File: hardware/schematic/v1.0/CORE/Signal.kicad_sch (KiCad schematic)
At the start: 13 parts, among them J2 Conn_Coaxial, J26 Conn_01x04_Socket, J3 Conn_Coaxial, J4 Conn_Coaxial, J5 Conn_Coaxial, U10 IPEX1, U11 IPEX1, U4 IPEX1, U8 IPEX1, U9 IPEX1

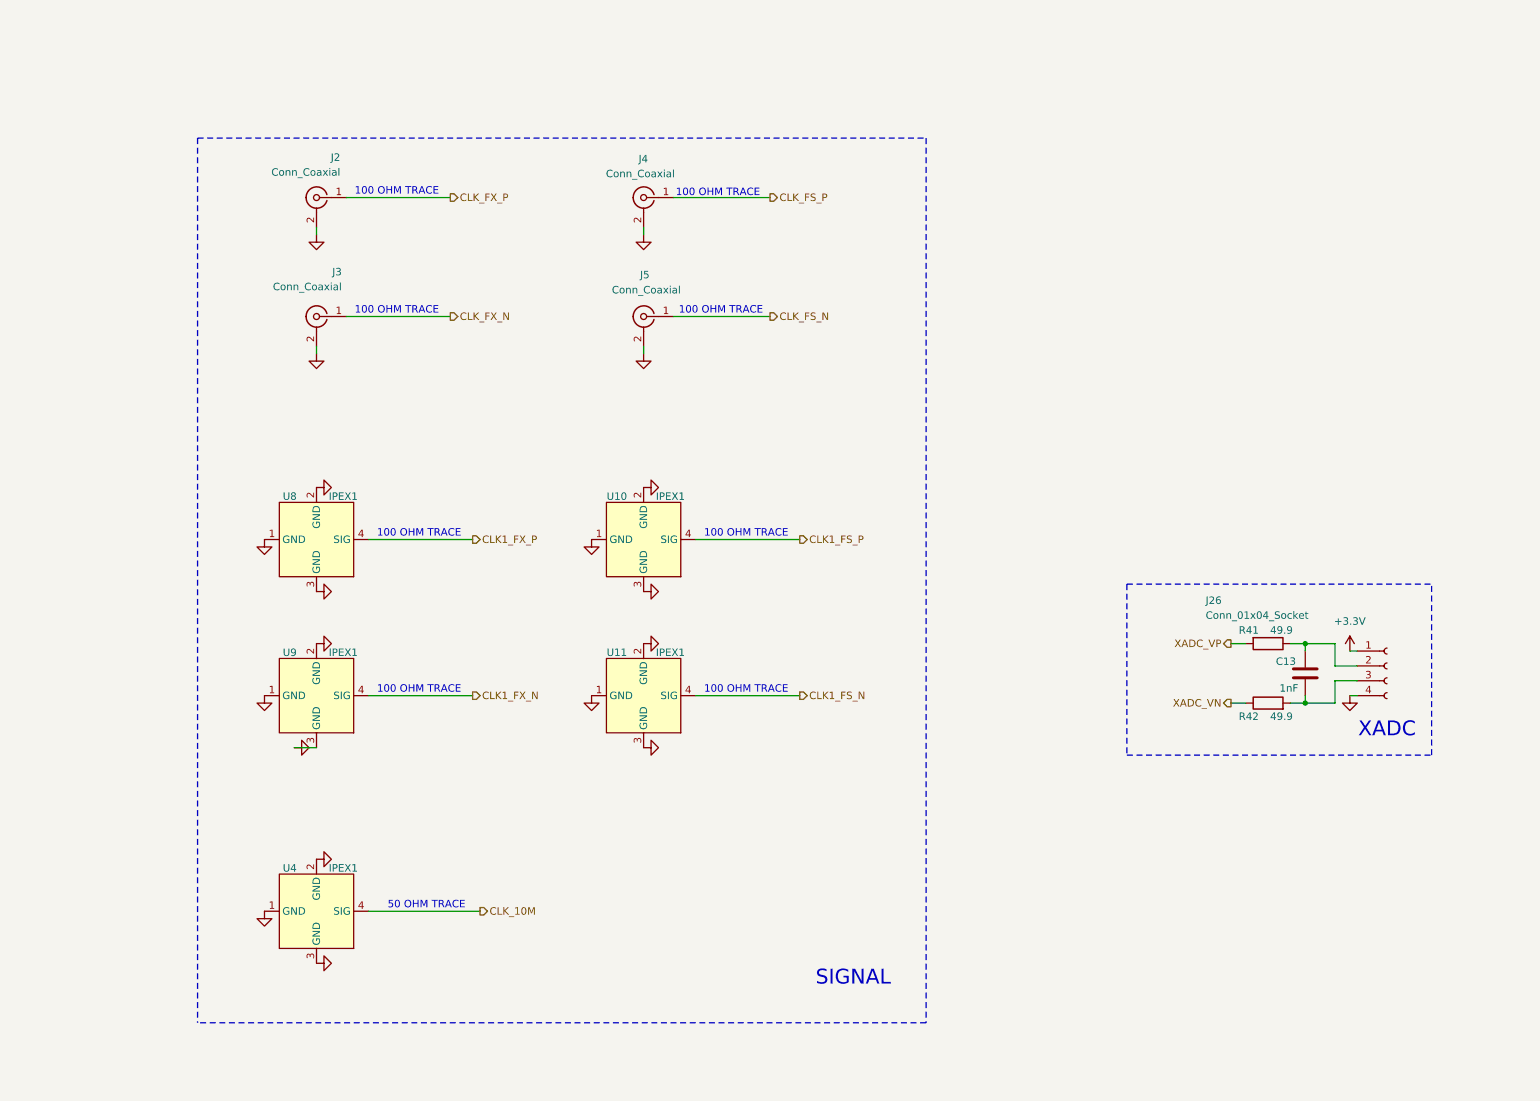
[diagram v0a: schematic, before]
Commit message: sch update
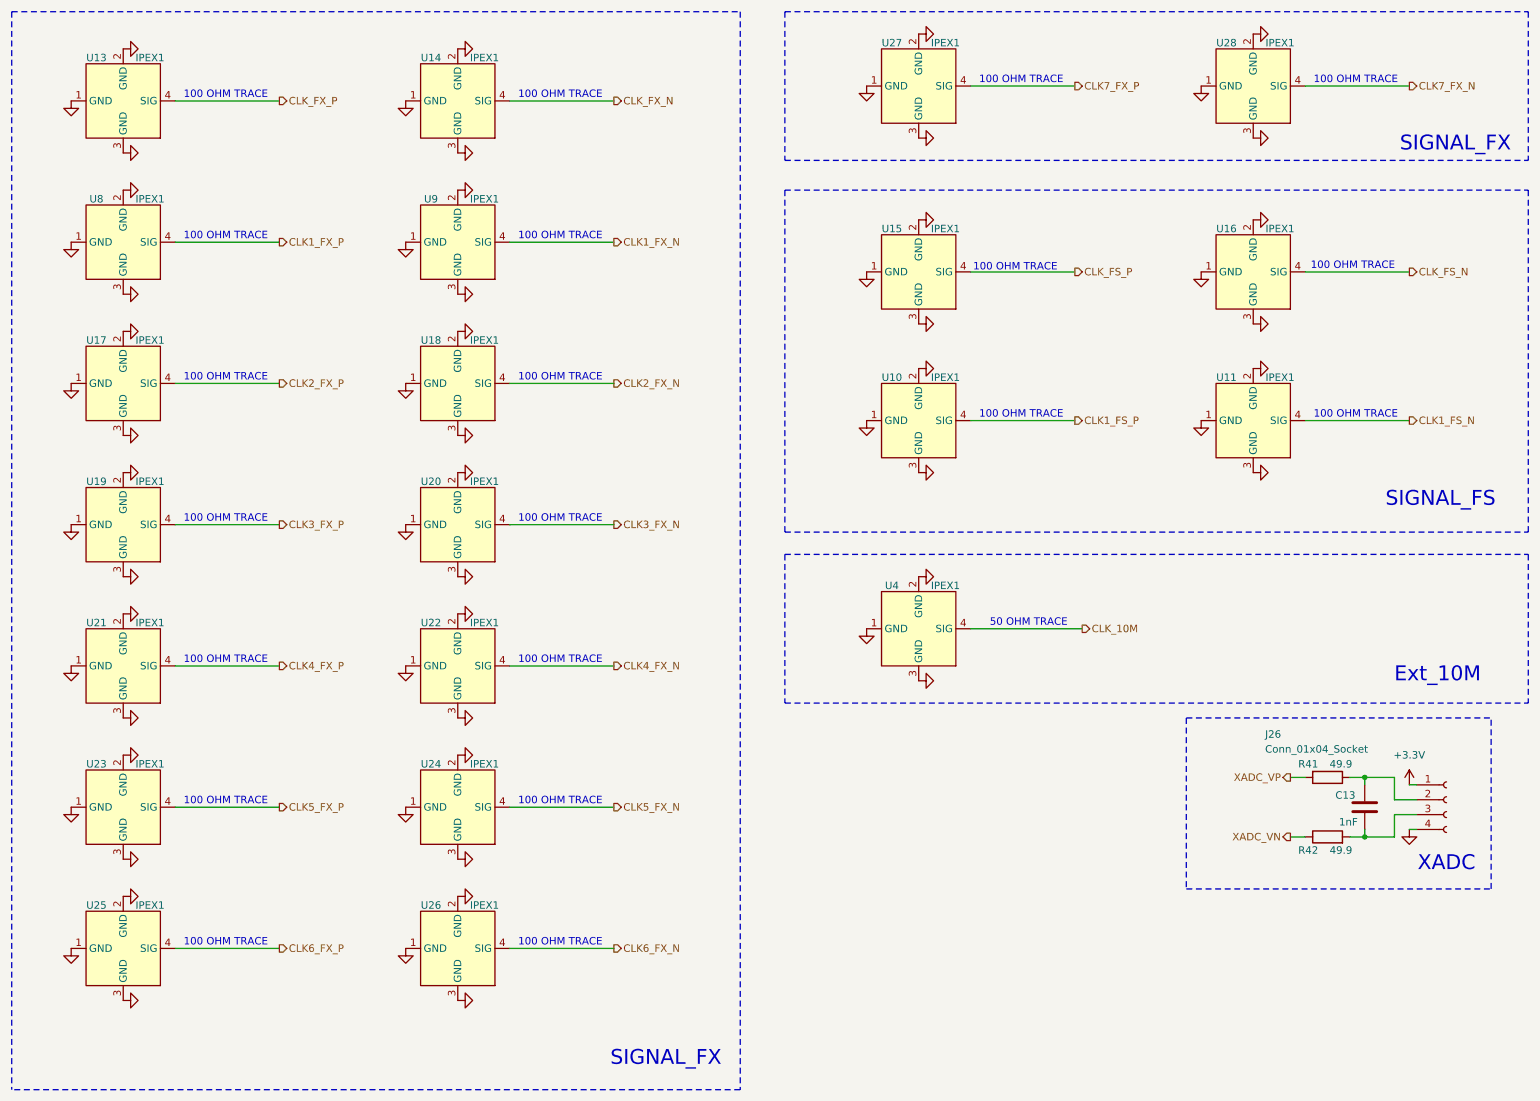
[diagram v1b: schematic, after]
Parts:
- removed J2, J3, J4, J5: Conn_Coaxial, Connector_Coaxial:SMA_Amphenol_132289_EdgeMount, symbol Connector:Conn_Coaxial
- added U13, U14, U15, U16, U17, U18, U19, U20, U21, U22, U23, U24, U25, U26, U27, U28: IPEX1, Counter:JLC_IPEX-1, symbol Counter:IPEX1
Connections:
- net CLK_FS_N: now also U16.4 (SIG)
- net CLK_FS_P: now also U15.4 (SIG)
- net CLK_FX_N: now also U14.4 (SIG)
- net CLK_FX_P: now also U13.4 (SIG)
- net GND: now also U13.1 (GND), U13.2 (GND), U13.3 (GND), U14.1 (GND), U14.2 (GND), U14.3 (GND), U15.1 (GND), U15.2 (GND), U15.3 (GND), U16.1 (GND), U16.2 (GND), U16.3 (GND), U17.1 (GND), U17.2 (GND), U17.3 (GND), U18.1 (GND), U18.2 (GND), U18.3 (GND), U19.1 (GND), U19.2 (GND), U19.3 (GND), U20.1 (GND), U20.2 (GND), U20.3 (GND), U21.1 (GND), U21.2 (GND), U21.3 (GND), U22.1 (GND), U22.2 (GND), U22.3 (GND), U23.1 (GND), U23.2 (GND), U23.3 (GND), U24.1 (GND), U24.2 (GND), U24.3 (GND), U25.1 (GND), U25.2 (GND), U25.3 (GND), U26.1 (GND), U26.2 (GND), U26.3 (GND), U27.1 (GND), U27.2 (GND), U27.3 (GND), U28.1 (GND), U28.2 (GND), U28.3 (GND)
- new net CLK2_FX_N: U18.4 (SIG)
- new net CLK2_FX_P: U17.4 (SIG)
- new net CLK3_FX_N: U20.4 (SIG)
- new net CLK3_FX_P: U19.4 (SIG)
- new net CLK4_FX_N: U22.4 (SIG)
- new net CLK4_FX_P: U21.4 (SIG)
- new net CLK5_FX_N: U24.4 (SIG)
- new net CLK5_FX_P: U23.4 (SIG)
- new net CLK6_FX_N: U26.4 (SIG)
- new net CLK6_FX_P: U25.4 (SIG)
- new net CLK7_FX_N: U28.4 (SIG)
- new net CLK7_FX_P: U27.4 (SIG)
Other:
- note added: "Ext_10M"
- note added: "SIGNAL_FS"
- note added: "SIGNAL_FX"
- note removed: "SIGNAL"
- moved on the sheet: C13, J26, R41, R42, U10, U11, U4, U8, U9
